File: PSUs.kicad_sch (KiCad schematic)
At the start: 27 parts, among them J2 Barrel_Jack, J6 SS-52400-004, U3 HUSB238_xxxDD, U4 AP62300WU-7, U8 AP62300WU-7

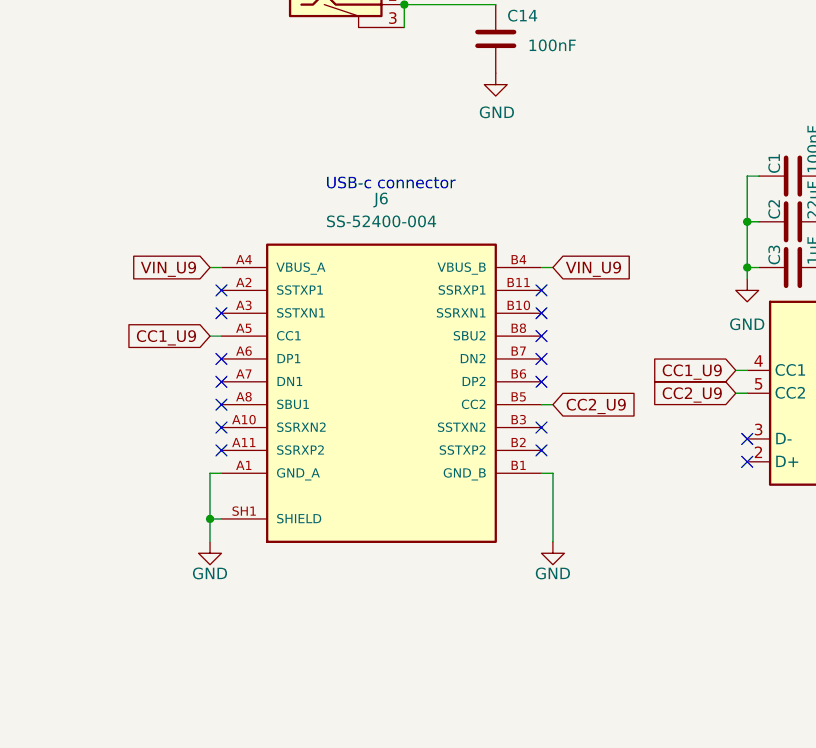
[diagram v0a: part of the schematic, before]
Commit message: Added lots and lots of traces in PCB design.
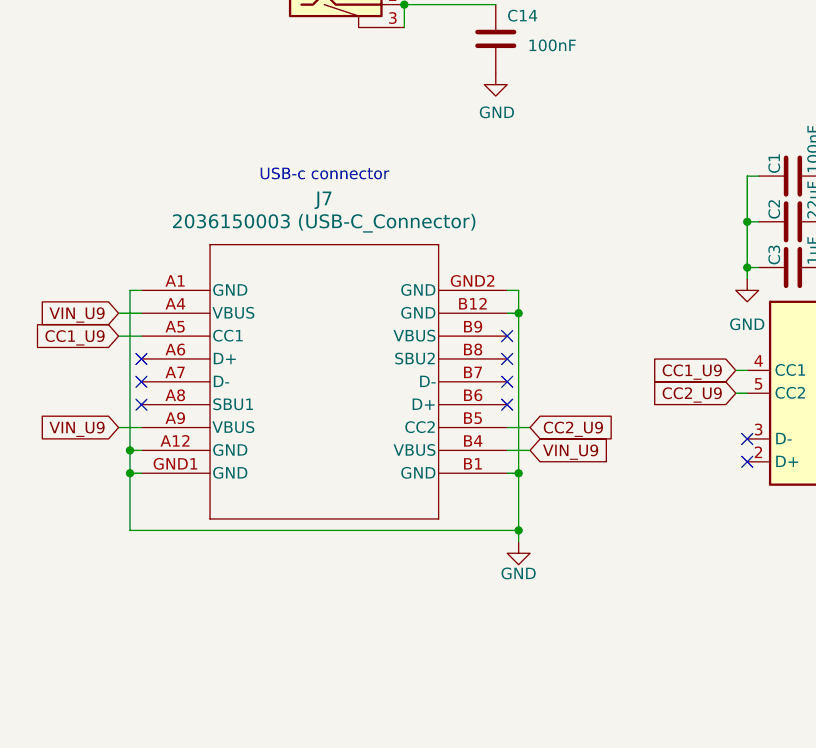
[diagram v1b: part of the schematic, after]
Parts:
- removed J6: SS-52400-004, SS-52400-004 (USB-c connector):STEWART_SS-52400-004 (USB-C), symbol SS-52400-004:SS-52400-004
- added J7: 2036150003 (USB-C_Connector), USB-C:CONN_2036150003_MOL(USB-c_connector), symbol 2026-03-08_10-34-21:2036150003
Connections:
- net CC1_U9: now also J7.A5 (CC1)
- net CC2_U9: now also J7.B5 (CC2)
- net GND: now also J7.A1 (GND), J7.A12 (GND), J7.B1 (GND), J7.B12 (GND), J7.GND1 (GND), J7.GND2 (GND)
- net VBUS_A renamed VIN_U9
- net VIN_U9: now also J7.A4 (VBUS), J7.A9 (VBUS), J7.B4 (VBUS)
- no-connect marks 21 -> 14
